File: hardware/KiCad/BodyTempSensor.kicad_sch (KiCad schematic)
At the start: 82 parts, among them IC3 TMP117MAIDRVT, IC4 TMP117MAIDRVT, IC5 TMP117MAIDRVT, IC6 TMP117MAIDRVT, IC7 NRF54L15-QFAA-R, J1 USB_C_Receptacle_USB2.0, J3 BAT, J6 Conn_02x05_Odd_Even, Q1 NMOS, Q2 NMOS, U3 MCP73833-xxx-UN, U4 TLV62568DBVR, U5 MCP6001-OT, Y1 32MHz

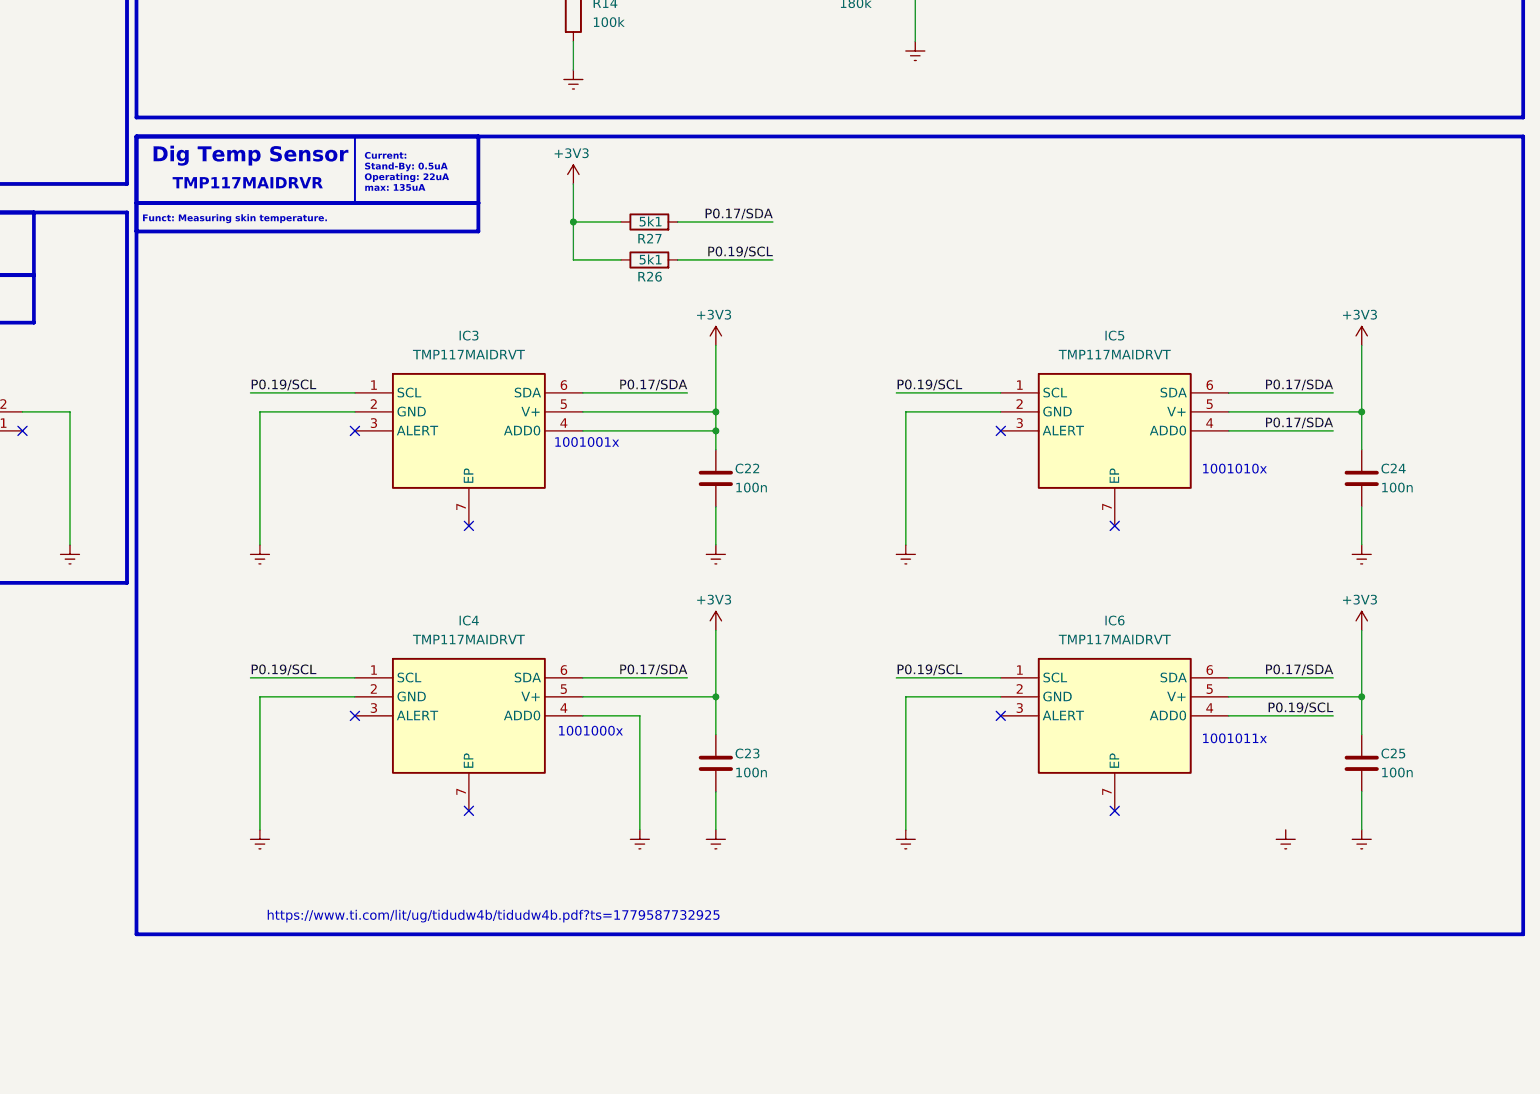
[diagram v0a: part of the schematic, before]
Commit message: testing
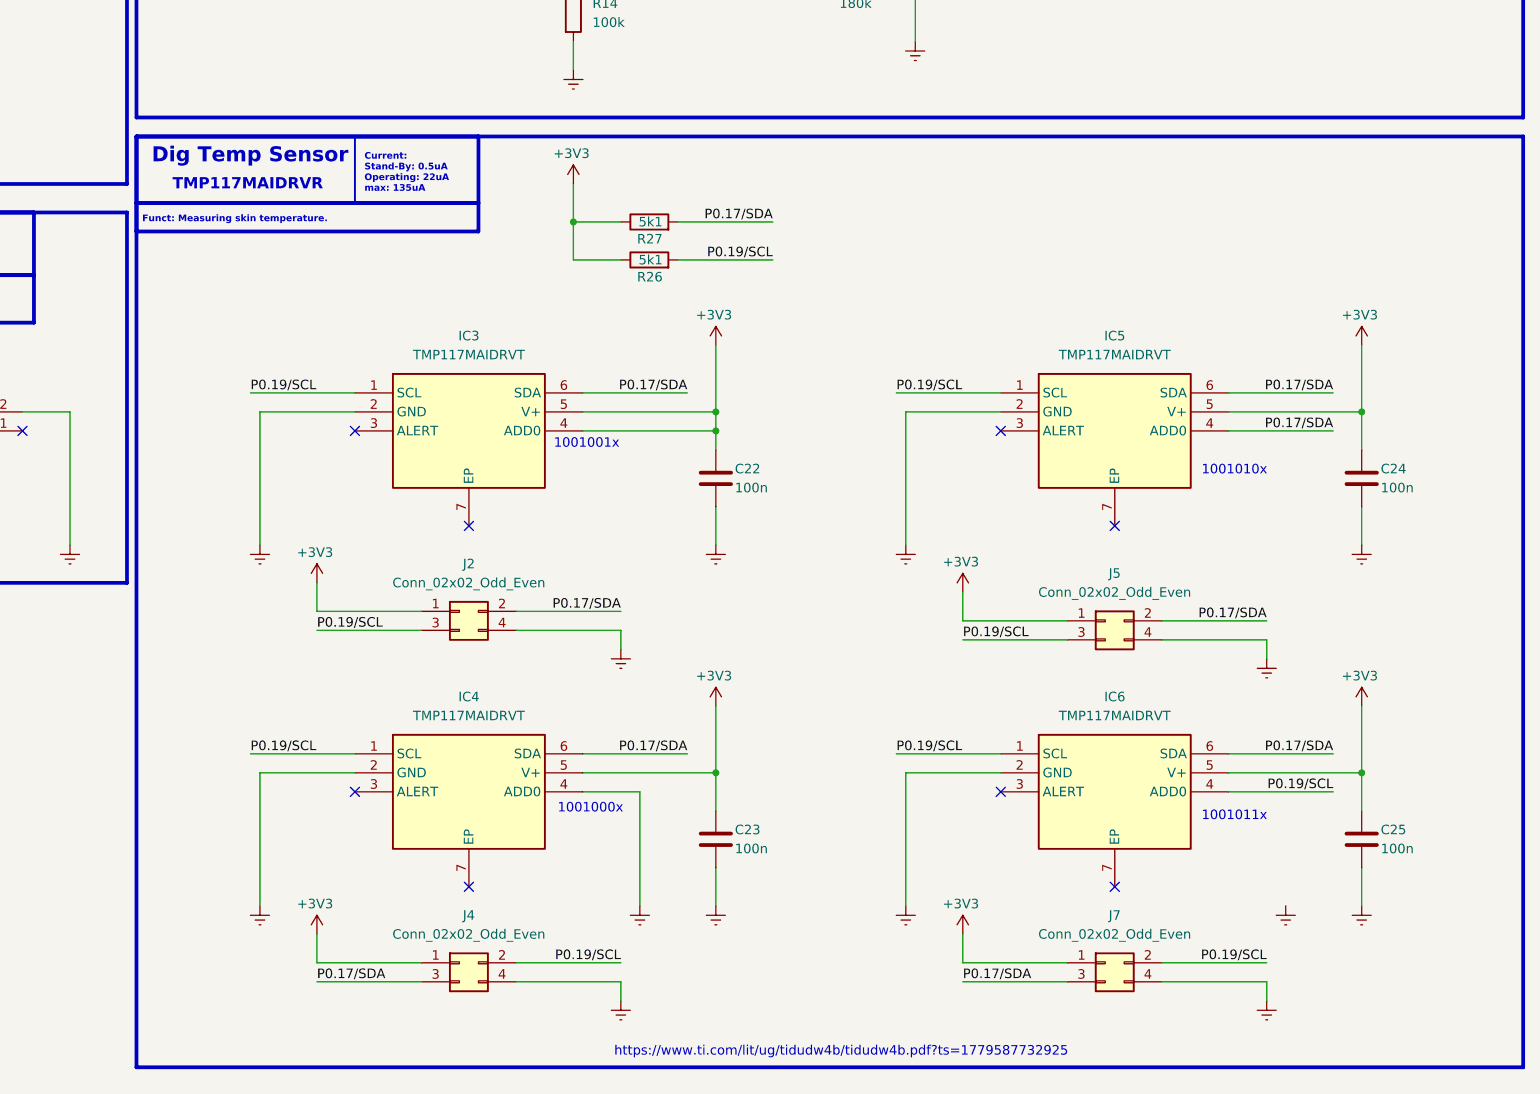
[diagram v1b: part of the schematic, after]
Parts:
- added J2, J5: Conn_02x02_Odd_Even, Connector_PinHeader_1.27mm:PinHeader_2x02_P1.27mm_Vertical_SMD, symbol Connector_Generic:Conn_02x02_Odd_Even
- added J4, J7: Conn_02x02_Odd_Even, Connector_PinHeader_1.27mm:PinHeader_2x02_P1.27mm_Vertical, symbol Connector_Generic:Conn_02x02_Odd_Even
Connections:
- net +3V3: now also J2.1 (Pin_1), J4.1 (Pin_1), J5.1 (Pin_1), J7.1 (Pin_1)
- net Earth: now also J2.4 (Pin_4), J4.4 (Pin_4), J5.4 (Pin_4), J7.4 (Pin_4)
- net P0.17/SDA: now also J2.2 (Pin_2), J4.3 (Pin_3), J5.2 (Pin_2), J7.3 (Pin_3)
- net P0.19/SCL: now also J2.3 (Pin_3), J4.2 (Pin_2), J5.3 (Pin_3), J7.2 (Pin_2)
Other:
- moved on the sheet: C23, C25, IC4, IC6
